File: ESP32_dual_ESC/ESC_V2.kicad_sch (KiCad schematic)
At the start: 37 parts, among them J1 A, J2 B, J3 C, Q1 HYG025N06LS1C2, Q2 HYG025N06LS1C2, Q3 HYG025N06LS1C2, Q4 HYG025N06LS1C2, Q5 HYG025N06LS1C2, Q6 HYG025N06LS1C2, U1 LM324, U11 DRV8300N

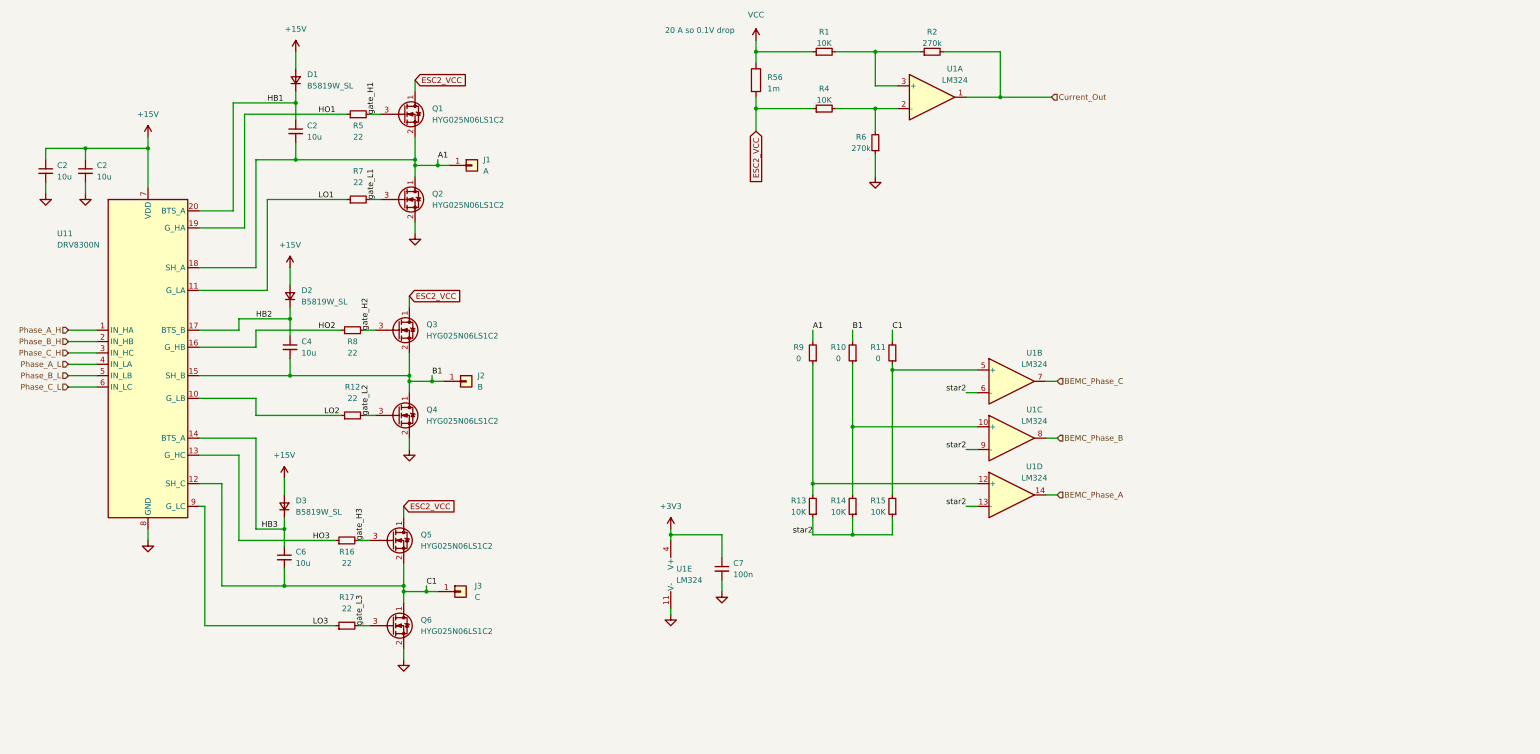
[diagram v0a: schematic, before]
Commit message: g
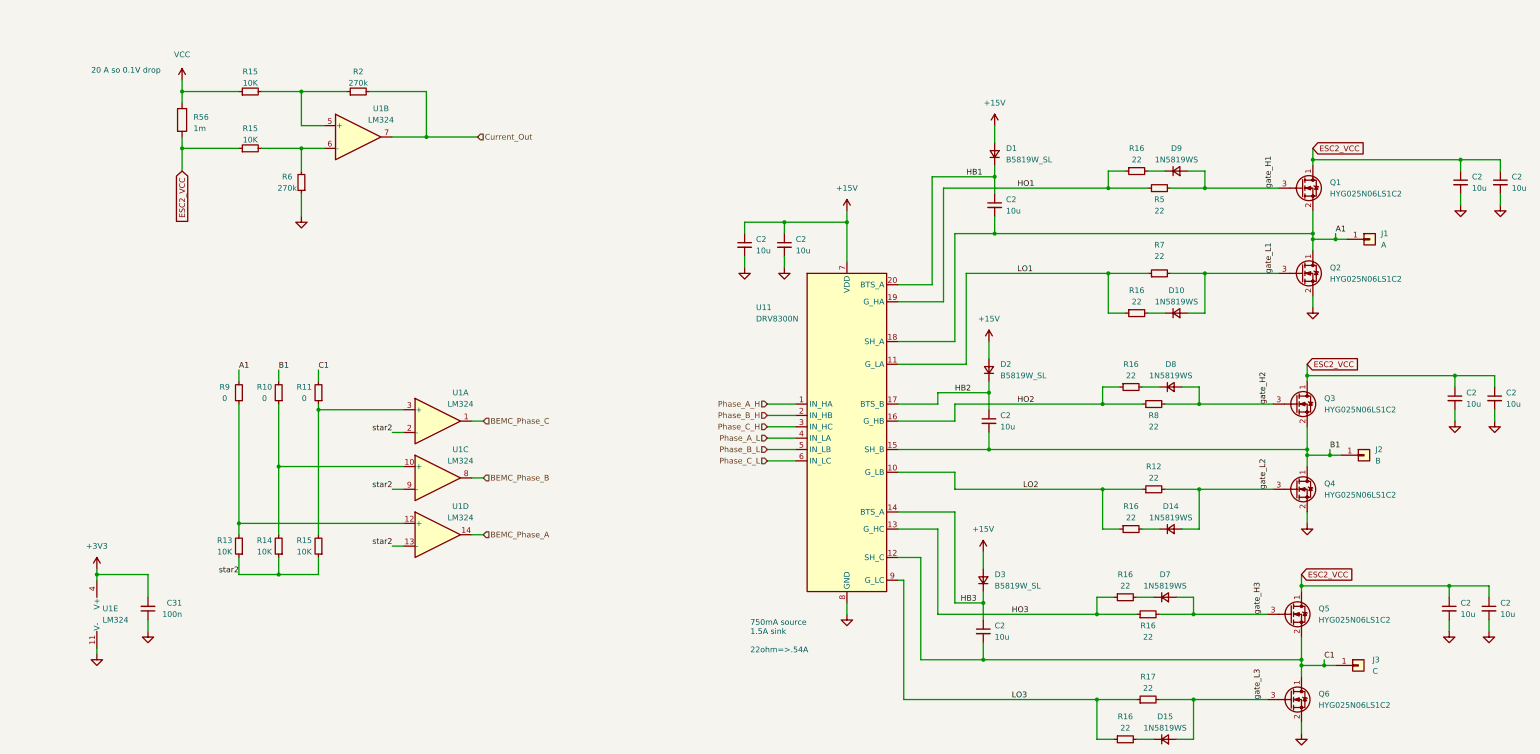
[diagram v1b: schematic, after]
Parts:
- removed C4, C6: 10u, Capacitor_SMD:C_0603_1608Metric, symbol Device:C_Small
- removed C7: 100n, symbol Device:C_Small
- removed R1, R4: 10K, symbol Device:R_Small
- added C2 (x6): 10u, Capacitor_SMD:C_1206_3216Metric, symbol Device:C_Small
- added C2 (x2): 10u, Capacitor_SMD:C_0805_2012Metric, symbol Device:C_Small
- added C31: 100n, Capacitor_SMD:C_0603_1608Metric, symbol Device:C_Small
- added D10, D14, D15, D7, D8, D9: 1N5819WS, Diode_SMD:D_SOD-323, symbol Device:D_Small
- added R15 (x2): 10K, Resistor_SMD:R_0603_1608Metric, symbol Device:R_Small
- added R16 (x6): 22, Resistor_SMD:R_0603_1608Metric, symbol Device:R_Small
- C2: footprint Capacitor_SMD:C_0603_1608Metric -> Capacitor_SMD:C_0805_2012Metric; LCSC C96446 -> C15850
- J1, J2, J3: footprint Mounting_Wuerth:Mounting_Wuerth_WA-SMSI-M1.6_H1.5mm_9774015633 -> MountingHole:MountingHole_2.5mm_Pad_TopBottom
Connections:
- net +3V3: now also C31.2
- net B1: now also C2.2
- net BEMC_Phase_C: now also U1.1; no longer U1.7
- net C1: now also C2.2
- net Current_Out: now also U1.7; no longer U1.1
- net ESC2_VCC: now also C2.1, C2.1, C2.1, C2.1, C2.1, C2.1, R15.1
- net GND: now also C2.2, C2.2, C2.2, C2.2, C2.2, C2.2, C31.1
- net HB2: now also C2.1
- net HB3: now also C2.1
- net HO1: now also R16.1
- net HO2: now also R16.1
- net HO3: now also R16.1
- net LO1: now also R16.1
- net LO2: now also R16.1
- net LO3: now also R16.1
- net VCC: now also R15.1
- net gate_H1: now also D9.2 (A)
- net gate_H2: now also D8.2 (A)
- net gate_H3: now also D7.2 (A)
- net gate_L1: now also D10.2 (A)
- net gate_L2: now also D14.2 (A)
- net gate_L3: now also D15.2 (A)
- net star2: now also U1.2 (-); no longer U1.6 (-)
- net at R2.1: now also U1.5 (+), R15.2; no longer U1.3 (+)
- net at R11.1, R15.2: now also U1.3 (+); no longer U1.5 (+)
- net at R6.2: now also U1.6 (-), R15.2; no longer U1.2 (-)
- new net: D15.1 (K), R16.2
- new net: D10.1 (K), R16.2
- new net: D14.1 (K), R16.2
- new net: D9.1 (K), R16.2
- new net: D7.1 (K), R16.2
- new net: D8.1 (K), R16.2
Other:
- note added: "750mA source 1.5A sink 22ohm=>.54A"
- moved on the sheet: C2, D1, D2, D3, J1, J2, J3, Q1, Q2, Q3, Q4, Q5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
